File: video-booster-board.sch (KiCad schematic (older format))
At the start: 139 parts, among them IC1 INA180A1IDBVT, J1 0473460001, J10 M20-9990246, J12 solder_jumper, J13 solder_jumper, J14 solder_jumper, J2 CHDMI-AMSS-01-C-Vertical, J3 CHDMI-AMSS-01-C-Vertical, J5 solder_jumper, J6 685119134923_, J7 solder_jumper, J8 solder_jumper, J9 685119134923_, SW1 1571983-5, U1 PTN3363, U2 TPS2110APW, U3 PTN3363, U4 LP2985-33DBVR, U5 NTS0102GT, U6 EFM32HG322F64, U7 NTS0102GT

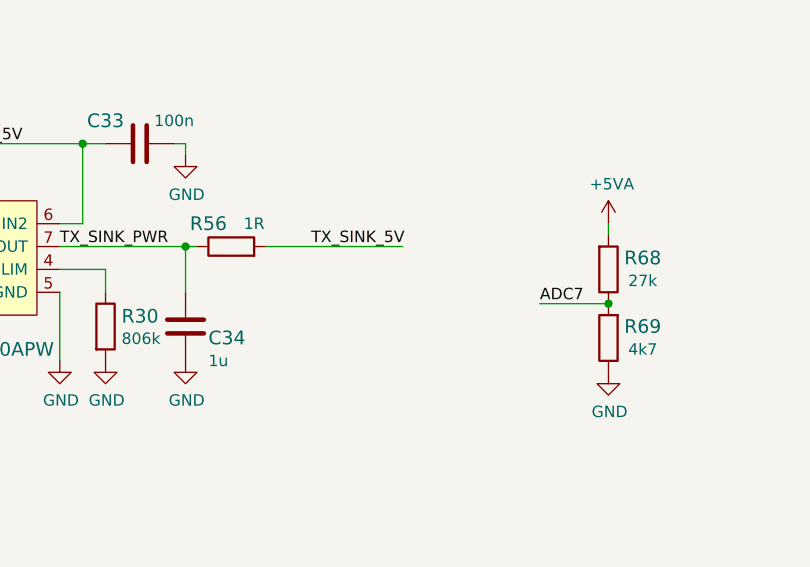
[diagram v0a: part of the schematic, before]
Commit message: Added BOM, schematic and gerbers for release 1.1
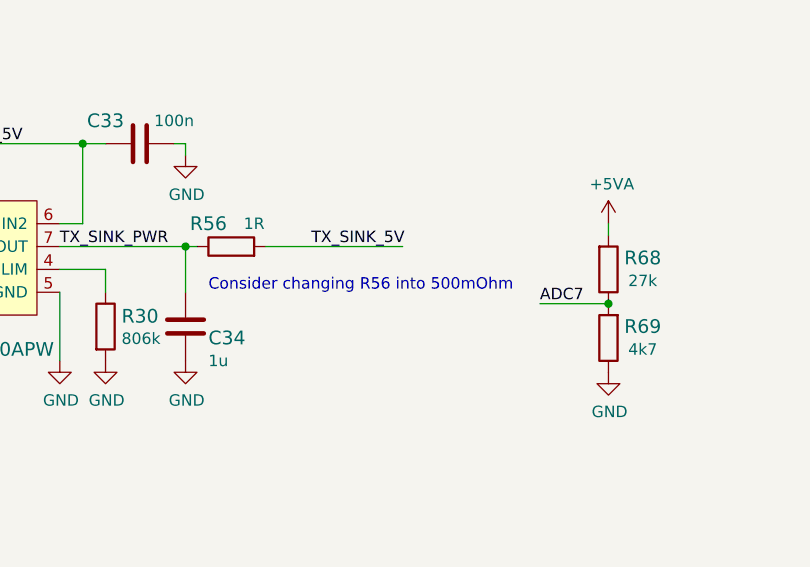
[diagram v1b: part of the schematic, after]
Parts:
- IC1: MPN (none) -> INA180A1IDBVT; Manufacturer (none) -> Texas Instruments
- J2, J3: footprint video-booster-board-footprints:CHDMI-AMSS-01-C-Vertical-mod1 -> video-booster-board-footprints:CHDMI-AMSS-01-C-Vertical; MPN (none) -> CHDMI-AMSX-01-X; Manufacturer (none) -> Kaweei
- J6, J9: MPN (none) -> 685119134923; Manufacturer (none) -> Wurth Elektronik
- SW1: Field10 1571983-5 -> (none); Field11 https://www.digikey.pl/product-detail/en/te-connectivity-al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 -> (none); Field12 1571983-5 -> (none); Field13 GDH04STR04=DIP SWITCH -> (none); Field14 DIP -> (none); Field4 450-1762-6-ND -> (none); Field5 Single Pole - Single Throw -> (none); Field6 .1 A -> (none); Field7 DIP-4 TE Connectivity -> (none); Field8 50 VDC -> (none); Field9 https://www.te.com/usa-en/product-1571983-5.html?te_bu=Cor&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 -> (none); MPN (none) -> 1571983-5; Manufacturer (none) -> TE Connectivity
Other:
- note added: "Consider changing R56 into 500mOhm"
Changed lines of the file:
@@
 EESchema Schematic File Version 4
+LIBS:video-booster-board-cache
 EELAYER 30 0
 EELAYER END
@@
 F 2 "video-booster-board-footprints:SOT-23-5" H 10550 6700 50  0001 C CNN
 F 3 "http://www.ti.com/lit/ds/symlink/ina180.pdf" H 10550 6700 50  0001 C CNN
+F 4 "Texas Instruments" H 10500 6150 50  0001 C CNN "Manufacturer"
+F 5 "INA180A1IDBVT" H 10500 6150 50  0001 C CNN "MPN"
 	1    10500 6150
 	1    0    0    -1
@@
 F 1 "1571983-5" H 14850 14776 50  0000 C CNN
 F 2 "video-booster-board-footprints:1571983-5" H 14850 14500 50  0001 L BNN
-F 3 "TE Connectivity" H 14850 14500 50  0001 L BNN
-F 4 "450-1762-6-ND" H 14850 14500 50  0001 L BNN "Field4"
-F 5 "Single Pole - Single Throw" H 14850 14500 50  0001 L BNN "Field5"
-F 6 ".1 A" H 14850 14500 50  0001 L BNN "Field6"
-F 7 "DIP-4 TE Connectivity" H 14850 14500 50  0001 L BNN "Field7"
-F 8 "50 VDC" H 14850 14500 50  0001 L BNN "Field8"
-F 9 "https://www.te.com/usa-en/product-1571983-5.html?te_bu=Cor&te_type=disp&te_campaign=seda_glo_cor-seda-global-disp-prtnr-fy19-seda-model-bom-cta_sma-317_1&elqCampaignId=32493" H 14850 14500 50  0001 L BNN "Field9"
-F 10 "1571983-5" H 14850 14500 50  0001 L BNN "Field10"
-F 11 "https://www.digikey.pl/product-detail/en/te-connectivity-alcoswitch-switches/1571983-5/450-1762-6-ND/2755727?utm_source=snapeda&utm_medium=aggregator&utm_campaign=symbol" H 14850 14500 50  0001 L BNN "Field11"
-F 12 "1571983-5" H 14850 14500 50  0001 L BNN "Field12"
-F 13 "GDH04STR04=DIP SWITCH" H 14850 14500 50  0001 L BNN "Field13"
-F 14 "DIP" H 14850 14500 50  0001 L BNN "Field14"
+F 3 "https://www.te.com/commerce/DocumentDelivery/DDEController?Action=srchrtrv&DocNm=1571983&DocType=Customer+Drawing&DocLang=English" H 14850 14500 50  0001 L BNN
+F 4 "TE Connectivity" H 14850 14500 50  0001 L BNN "Manufacturer"
+F 5 "1571983-5" H 14850 14500 50  0001 L BNN "MPN"
 	1    14850 14500
 	1    0    0    -1
@@
 F 1 "685119134923_" V 10800 2250 50  0000 L CNN
 F 2 "video-booster-board-footprints:HDMI_A_Female_685119134923" H 10550 3450 60  0001 L CNN
-F 3 "https://katalog.we-online.de/em/datasheet/685119134923.pdf" H 10375 3250 50  0001 C CNN
+F 3 "https://www.we-online.com/catalog/datasheet/685119134923.pdf" H 10375 3250 50  0001 C CNN
+F 4 "Wurth Elektronik" H 10350 3250 50  0001 C CNN "Manufacturer"
+F 5 "685119134923" H 10350 3250 50  0001 C CNN "MPN"
 	1    10350 3250
 	1    0    0    -1
@@
 F 1 "685119134923_" V 11200 9700 50  0000 L CNN
 F 2 "video-booster-board-footprints:HDMI_A_Female_685119134923" H 10950 10900 60  0001 L CNN
-F 3 "https://katalog.we-online.de/em/datasheet/685119134923.pdf" H 10775 10700 50  0001 C CNN
+F 3 "https://www.we-online.com/catalog/datasheet/685119134923.pdf" H 10775 10700 50  0001 C CNN
+F 4 "685119134923" H 10750 10700 50  0001 C CNN "MPN"
+F 5 "Wurth Elektronik" H 10750 10700 50  0001 C CNN "Manufacturer"
 	1    10750 10700
 	1    0    0    -1
@@
 F 0 "J2" V 1650 2700 50  0000 R CNN
 F 1 "CHDMI-AMSS-01-C-Vertical" V 1750 3700 50  0000 R CNN
-F 2 "video-booster-board-footprints:CHDMI-AMSS-01-C-Vertical-mod1" H 2300 3600 60  0001 L CNN
+F 2 "video-booster-board-footprints:CHDMI-AMSS-01-C-Vertical" H 2300 3600 60  0001 L CNN
 F 3 "" H 2175 3550 50  0001 C CNN
+F 4 " CHDMI-AMSX-01-X" H 2100 3400 50  0001 C CNN "MPN"
+F 5 "Kaweei" H 2100 3400 50  0001 C CNN "Manufacturer"
 	1    2100 3400
 	1    0    0    -1
@@
 F 0 "J3" V 2000 10150 50  0000 R CNN
 F 1 "CHDMI-AMSS-01-C-Vertical" V 2100 11150 50  0000 R CNN
-F 2 "video-booster-board-footprints:CHDMI-AMSS-01-C-Vertical-mod1" H 2650 11050 60  0001 L CNN
+F 2 "video-booster-board-footprints:CHDMI-AMSS-01-C-Vertical" H 2650 11050 60  0001 L CNN
 F 3 "" H 2525 11000 50  0001 C CNN
+F 4 " CHDMI-AMSX-01-X" H 2450 10850 50  0001 C CNN "MPN"
+F 5 "Kaweei" H 2450 10850 50  0001 C CNN "Manufacturer"
 	1    2450 10850
 	1    0    0    -1
@@
 	1    0    0    -1
 $EndComp
+Text Notes 16500 6150 0    50   ~ 0
+Consider changing R56 into 500mOhm
 $EndSCHEMATC
